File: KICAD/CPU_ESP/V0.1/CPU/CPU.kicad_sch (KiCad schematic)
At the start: 4 parts, among them J101 USB_B_Mini, J102 Conn_01x04, SW101 SW_Push_45deg, SW102 SW_Push_45deg

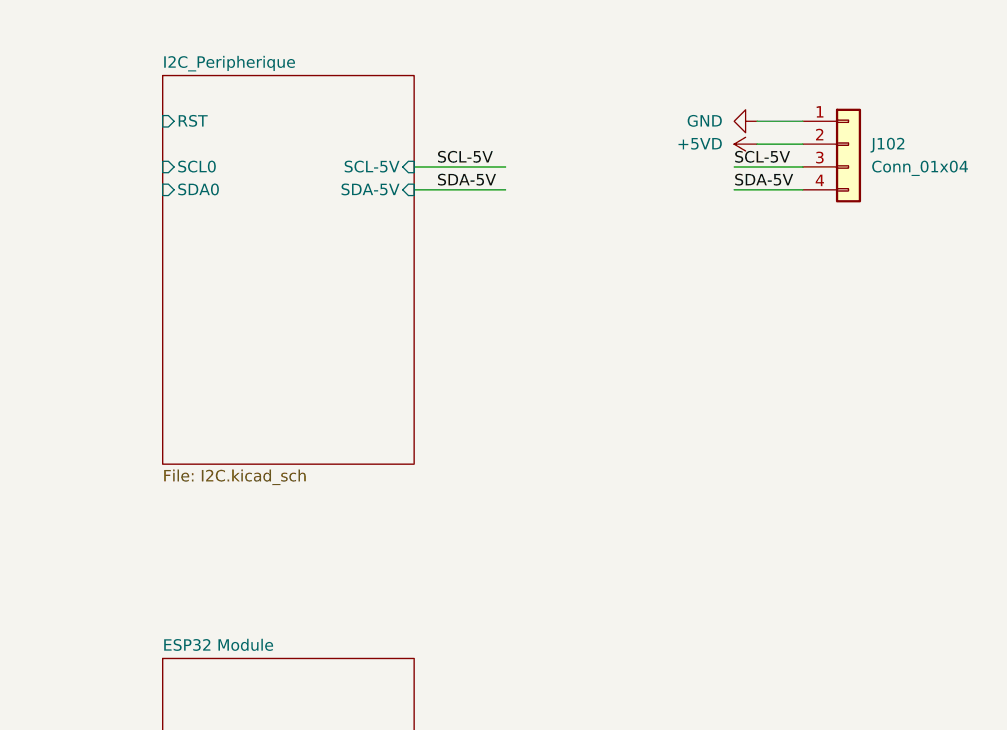
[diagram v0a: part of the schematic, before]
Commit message: Update
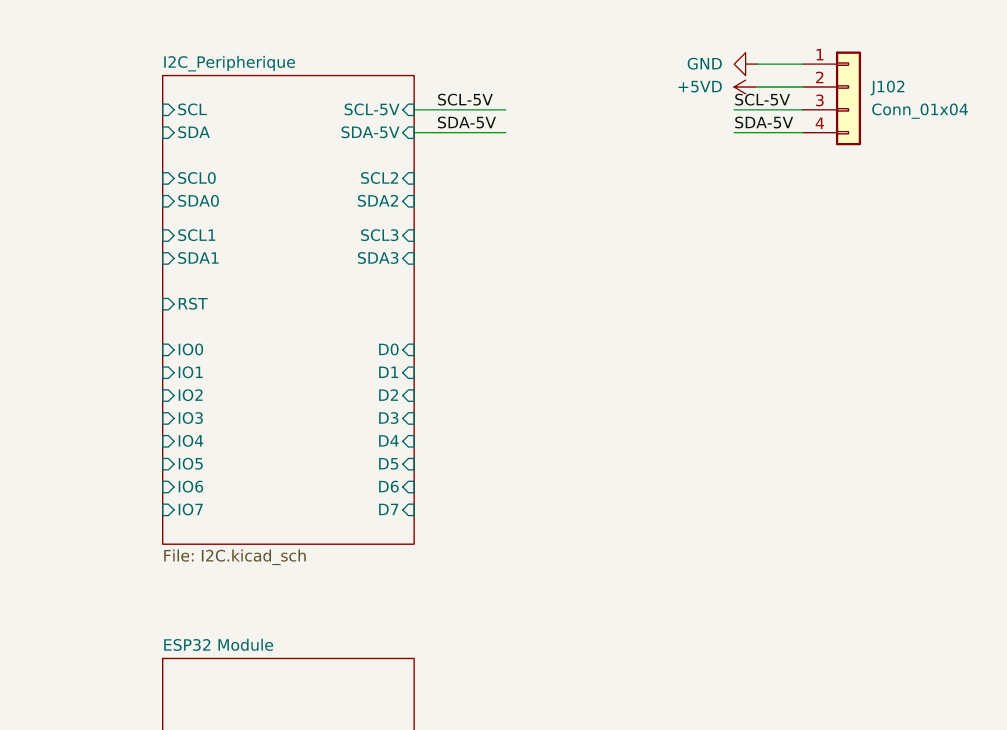
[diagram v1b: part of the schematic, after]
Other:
- sheet I2C_Peripherique ports: added D0, D1, D2, D3, D4, D5, D6, D7, IO0, IO1, IO2, IO3, IO4, IO5, IO6, IO7, SCL, SCL1, SCL2, SCL3, SDA, SDA1, SDA2, SDA3; removed none
- moved on the sheet: J102
